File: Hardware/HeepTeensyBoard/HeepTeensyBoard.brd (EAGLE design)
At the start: 100 x 80 mm, 31 parts, among them J1 MAGJACK, J4 POWER_JACKPTH, Q1 25MHz, U1 ENC28J60-SO

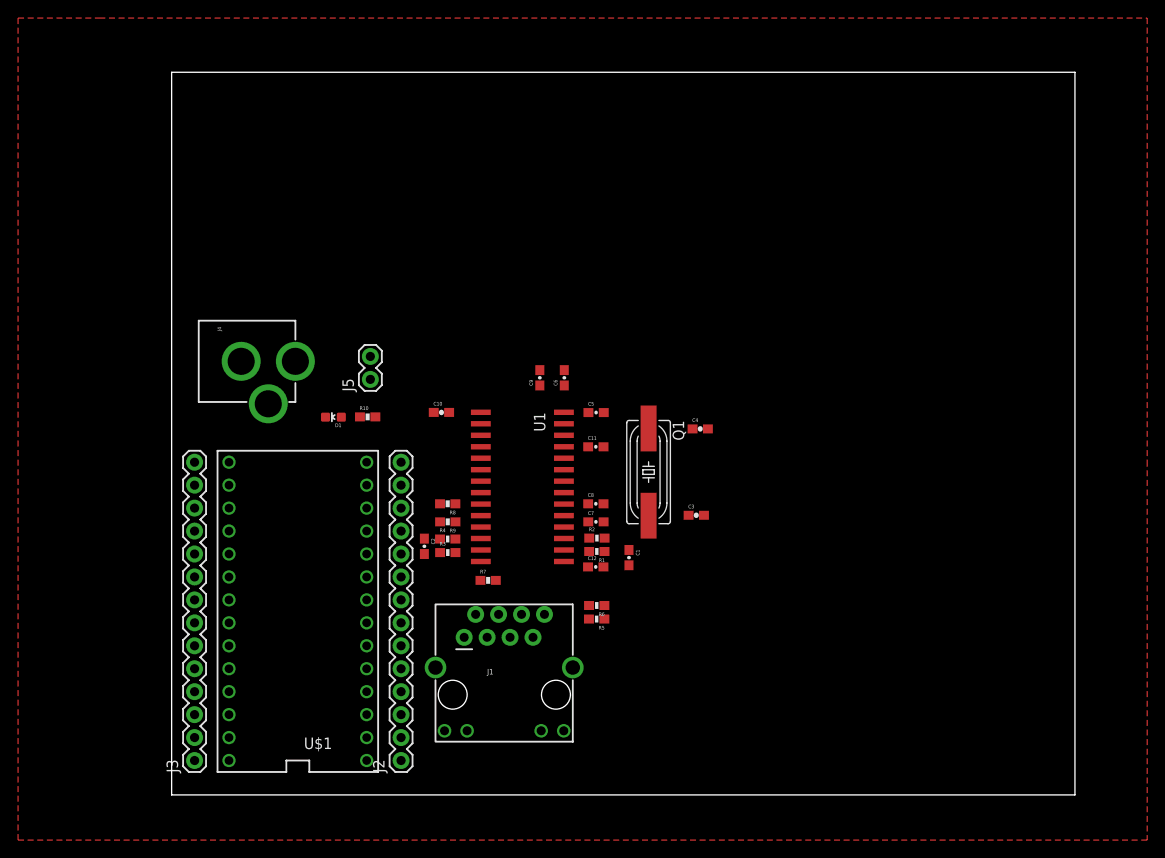
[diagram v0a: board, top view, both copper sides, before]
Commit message: #151 First full board layout
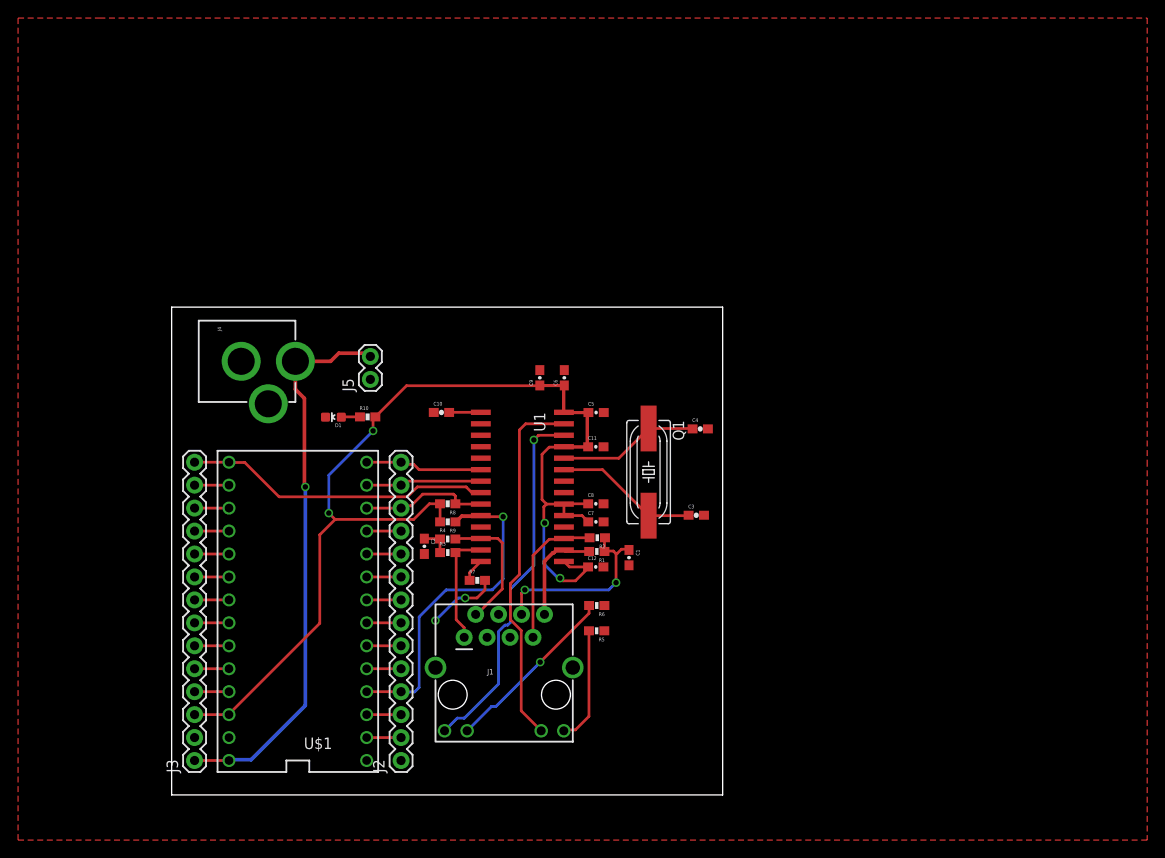
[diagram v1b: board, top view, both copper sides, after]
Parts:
- moved R5 1.30 mm to (47.0, 18.2)
- moved R7 1.20 mm to (33.8, 23.8)
- moved R2 0.06 mm to (47.1, 28.5), turned to 180 degrees
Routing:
- net 3.3V: track 0.00 -> 141.3 mm, vias 0 -> 4
- net VIN: track 0.00 -> 62.2 mm, vias 0 -> 1
- net #RESET: track 0.00 -> 41.1 mm, vias 0 -> 1
- net LEDB: track 0.00 -> 40.5 mm, vias 0 -> 1
- net LEDA: track 0.00 -> 40.3 mm
- net SCK: track 0.00 -> 34.0 mm
- net N$7: track 0.00 -> 21.1 mm, vias 0 -> 2
- net N$6: track 0.00 -> 19.7 mm, vias 0 -> 1
- net N$4: track 0.00 -> 16.1 mm
- net N$12: track 0.00 -> 15.9 mm
- net N$13: track 0.00 -> 15.6 mm
- net N$2: track 0.00 -> 14.6 mm
- net #CS: track 0.00 -> 14.2 mm
- net SO: track 0.00 -> 13.0 mm
- net N$10: track 0.00 -> 12.9 mm
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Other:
- board size 100 x 80 mm -> 61 x 54 mm
